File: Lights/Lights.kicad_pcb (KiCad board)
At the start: 2 copper layers, 102.5 x 200 mm, 100 parts, among them J101 chain_in, J102 chain_out, J103 Input1, J104 Input1, J105 Input1, J106 THRU, J107 THRU, J108 IN, J109 EuroPower, J110 ExternalPower, J401 Light, J701 Light, J801 Light, Q401 PN2222A, Q402 IRF540N, Q701 PN2222A, Q702 IRF540N, Q801 PN2222A, Q802 IRF540N, U101 L7805, U102 L7805, U201 TL074, U301 74LS04, U302 6N138, U401 6N138, U501 TL074, U601 TL074, U701 6N138, U801 6N138

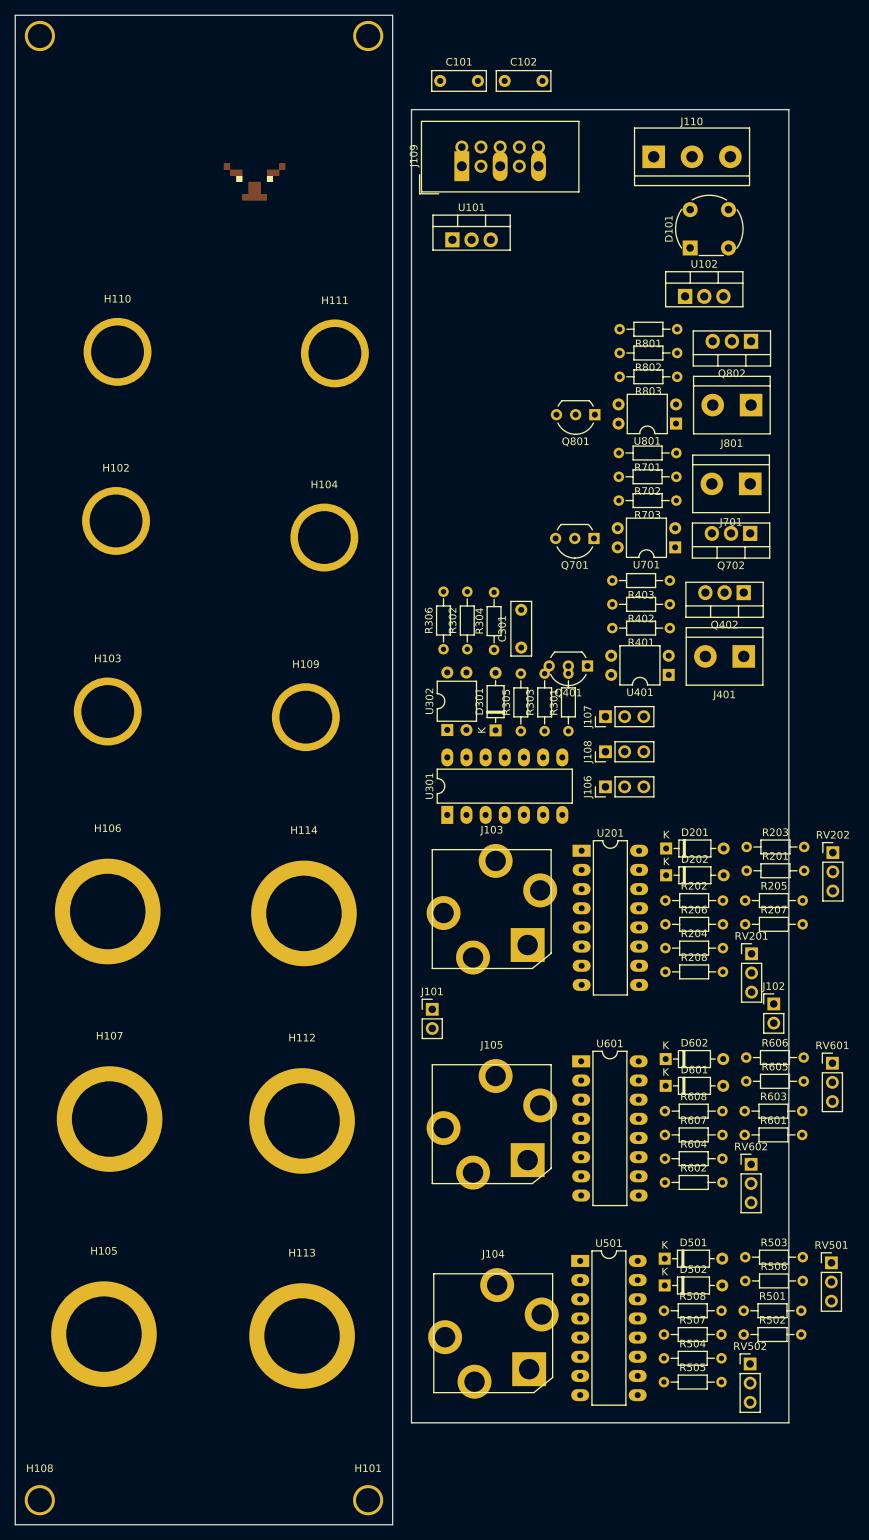
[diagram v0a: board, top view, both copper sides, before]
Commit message: Finished schematic and routing
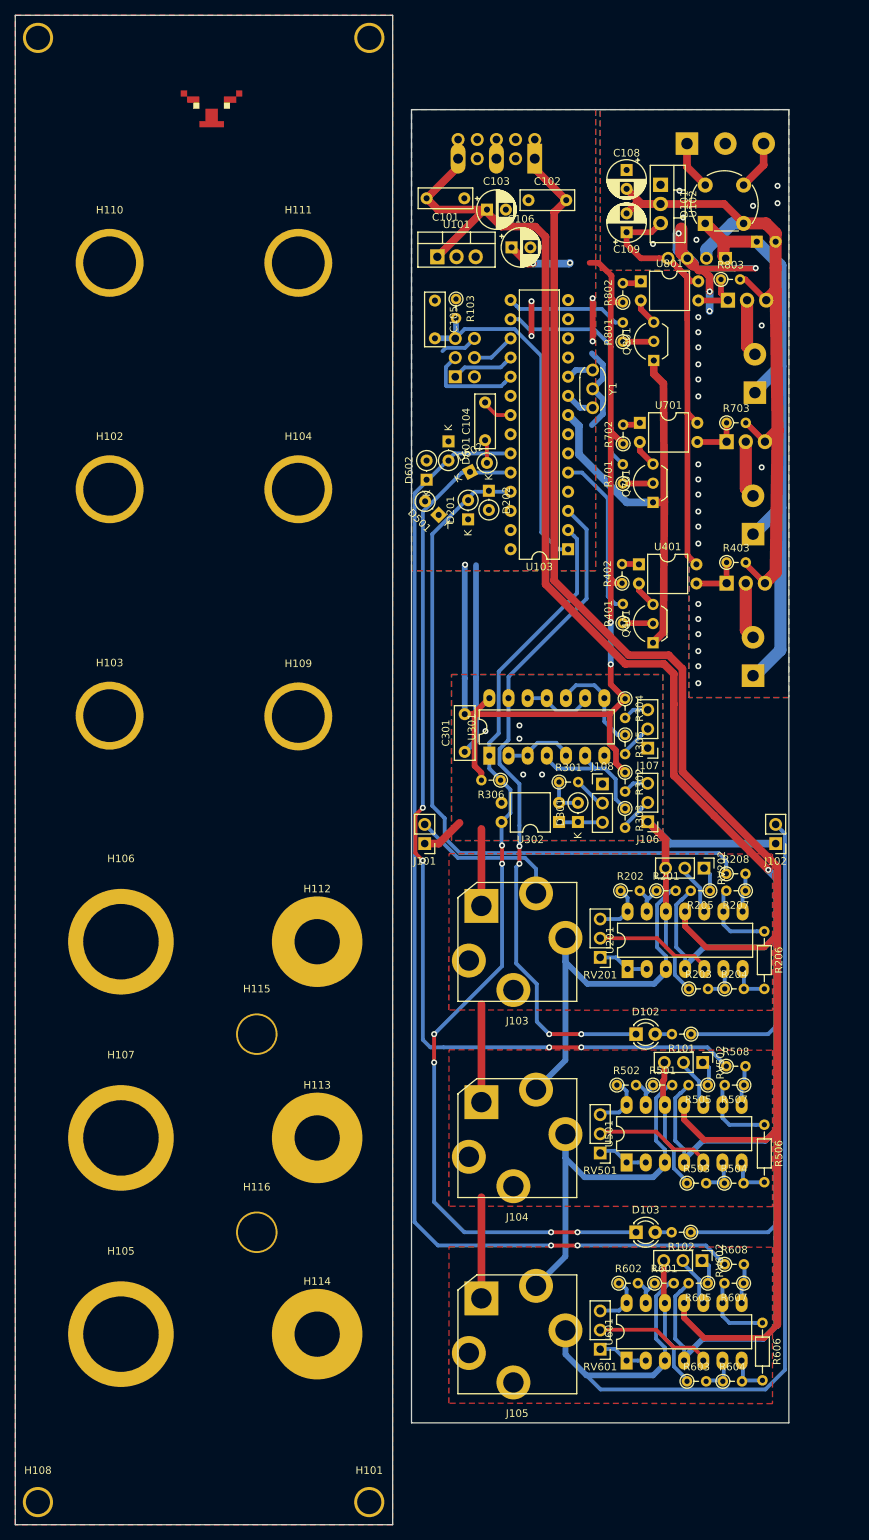
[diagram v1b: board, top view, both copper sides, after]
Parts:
- added C103: 1u, Capacitor_THT:CP_Radial_D5.0mm_P2.50mm, F.Cu at (74.5, 37.8)
- added C104: 100n, Capacitor_THT:C_Disc_D7.0mm_W2.5mm_P5.00mm, F.Cu at (74.2, 68.3)
- added C105: 100n, Capacitor_THT:C_Disc_D7.0mm_W2.5mm_P5.00mm, F.Cu at (67.6, 49.8)
- added C106: 1u, Capacitor_THT:CP_Radial_D5.0mm_P2.50mm, F.Cu at (77.8, 42.8)
- added C107: 10u, Capacitor_THT:CP_Radial_D5.0mm_P2.50mm, B.Cu at (110.2, 42.0)
- added C108: 1u, Capacitor_THT:CP_Radial_D5.0mm_P2.50mm, F.Cu at (93.0, 32.5)
- added C109: 1u, Capacitor_THT:CP_Radial_D5.0mm_P2.50mm, F.Cu at (93.0, 40.8)
- added D102: LED, LED_THT:LED_D3.0mm_FlatTop, F.Cu at (94.2, 147.0)
- added D103: LED, LED_THT:LED_D3.0mm_FlatTop, F.Cu at (94.2, 173.2)
- added H115: Led_Hole, Kosmo_panel:Kosmo_LED_Hole, F.Cu at (44.0, 147.0)
- added H116: Led_Hole, Kosmo_panel:Kosmo_LED_Hole, F.Cu at (44.0, 173.2)
- added J111: Programming, Connector_IDC:IDC-Header_2x03_P2.54mm_Vertical, B.Cu at (70.3, 59.9)
- added J112: chain_power, Connector_PinHeader_2.54mm:PinHeader_1x04_P2.54mm_Vertical, B.Cu at (106.1, 44.2)
- added R101: 1K, Resistor_THT:R_Axial_DIN0204_L3.6mm_D1.6mm_P2.54mm_Vertical, F.Cu at (101.5, 147.0)
- added R102: 1K, Resistor_THT:R_Axial_DIN0204_L3.6mm_D1.6mm_P2.54mm_Vertical, F.Cu at (101.5, 173.2)
- added R103: 22k, Resistor_THT:R_Axial_DIN0204_L3.6mm_D1.6mm_P2.54mm_Vertical, F.Cu at (70.4, 49.6)
- added U103: ATmega328P-PU, Package_DIP:DIP-28_W7.62mm, F.Cu at (85.2, 82.8)
- added Y1: 16MHz, Crystal:Resonator-3Pin_W6.0mm_H3.0mm, F.Cu at (88.5, 59.0)
- D201, D202, D301, D501, D502, D601, D602: footprint Diode_THT:D_DO-35_SOD27_P7.62mm_Horizontal -> Diode_THT:D_DO-35_SOD27_P2.54mm_Vertical_KathodeUp
- H112, H113, H114: footprint Kosmo_panel:Kosmo_Jack_Hole -> MountingHole:MountingHole_6mm_Pad
- J104: value Input1 -> Input2
- J105: value Input1 -> Input3
- J107: value THRU -> OUT
- J109, J110, J401, J701, J801, Q402, Q702, Q802: moved to B.Cu
- R201, R202, R203, R204, R205, R207, R208, R301, R302, R303, R304, R305, R306, R401, R402, R403, R501, R502, R503, R504, R505, R507, R508, R601, R602, R603, R604, R605, R607, R608, R701, R702, R703, R801, R802, R803: footprint Resistor_THT:R_Axial_DIN0204_L3.6mm_D1.6mm_P7.62mm_Horizontal -> Resistor_THT:R_Axial_DIN0204_L3.6mm_D1.6mm_P2.54mm_Vertical
- U201, U501, U601: footprint Package_DIP:DIP-16_W7.62mm_LongPads -> Package_DIP:DIP-14_W7.62mm_LongPads
- moved D502 110.8 mm to (72.2, 72.5), turned to 28 degrees
- moved D501 103.0 mm to (68.1, 78.2), turned to 135 degrees
- moved D601 90.1 mm to (69.4, 68.5), turned to 270 degrees
- moved D602 83.0 mm to (66.5, 73.5), turned to 90 degrees
- moved D202 56.1 mm to (74.8, 75.0), turned to 270 degrees
- moved H114 55.8 mm to (52.0, 186.8)
- moved D201 50.9 mm to (72.0, 78.8), turned to 90 degrees
- moved RV601 48.8 mm to (89.5, 188.8), turned to 180 degrees
- moved RV502 40.4 mm to (103.1, 150.8), turned to 270 degrees
- moved U601 40.1 mm to (93.0, 190.2), turned to 90 degrees
- moved R505 39.8 mm to (103.8, 153.8), turned to 180 degrees
- moved R502 37.1 mm to (91.7, 153.8)
- moved R603 36.6 mm to (101.0, 193.0)
- moved R606 35.2 mm to (111.0, 185.2), turned to 270 degrees
- moved R507 34.7 mm to (108.5, 153.8), turned to 180 degrees
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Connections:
- net /Normalize/Norm renamed /ADC1
- net /sheet606D2594/Norm renamed /ADC2
- net /sheet606D67AE/Norm renamed /ADC3
- J106 pad R: Net-(J106-PadR) -> /MIDI/MIDI_THRU-
- J106 pad S: Net-(J106-PadS) -> GND
- J106 pad T: Net-(J106-PadT) -> /MIDI/MIDI_THRU+
- J107 pad R: Net-(J107-PadR) -> /MIDI/MIDI_OUT-
- J107 pad S: Net-(J107-PadS) -> GND
- J107 pad T: Net-(J107-PadT) -> /MIDI/MIDI_OUT+
- J108 pad R: Net-(J108-PadR) -> /MIDI/MIDI_IN-
- J108 pad T: Net-(J108-PadT) -> /MIDI/MIDI_IN+
- Q402 pad 1: +5V -> Net-(Q402-Pad1)
- Q702 pad 1: +5V -> Net-(Q702-Pad1)
- Q802 pad 1: +5V -> Net-(Q802-Pad1)
- R401 pad 2: /Switching/PWM -> /PWM3
- R403 pad 1: Net-(R403-Pad1) -> Net-(Q402-Pad1)
- R701 pad 2: /sheet60725942/PWM -> /PWM2
- R703 pad 1: Net-(R703-Pad1) -> Net-(Q702-Pad1)
- R801 pad 2: /sheet607266DD/PWM -> /PWM1
- R803 pad 1: Net-(R803-Pad1) -> Net-(Q802-Pad1)
- U401 pad 3: Net-(R403-Pad1) -> Net-(Q402-Pad1)
- U401 pad 4: +5V -> +5VP
- U701 pad 3: Net-(R703-Pad1) -> Net-(Q702-Pad1)
- U701 pad 4: +5V -> +5VP
- U801 pad 3: Net-(R803-Pad1) -> Net-(Q802-Pad1)
- U801 pad 4: +5V -> +5VP
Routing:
- net +12V: track 0.00 -> 299.3 mm, vias 0 -> 1
- net GND: track 0.00 -> 233.3 mm, vias 0 -> 9
- net -12V: track 0.00 -> 223.3 mm
- net /ADC3: track 0.00 -> 154.9 mm, vias 0 -> 2
- net +5V: track 0.00 -> 140.3 mm, vias 0 -> 5
- net /sheet606D67AE/In: track 0.00 -> 135.7 mm
- net /MIDI_IN: track 0.00 -> 128.2 mm, vias 0 -> 6
- net /ADC2: track 0.00 -> 127.0 mm, vias 0 -> 4
- net -VDC: track 0.00 -> 97.7 mm
- net /ADC1: track 0.00 -> 93.9 mm
- net /MIDI_OUT: track 0.00 -> 89.7 mm, vias 0 -> 4
- net +VDC: track 0.00 -> 80.2 mm
- net +5VP: track 0.00 -> 62.0 mm
- net /Normalize/In: track 0.00 -> 52.7 mm
- net /sheet606D2594/In: track 0.00 -> 52.4 mm
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- added copper zone on F.Cu, net +5V
- added copper zone on B.Cu, net GND
- added copper zone on F.Cu, net GND
- added copper zone on B.Cu, net GNDPWR
- added copper zone on F.Cu, net GNDPWR
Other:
- net class Default: clearance 0.2 -> 0.127; trace_width 0.25 -> 0.127; via_dia 0.8 -> 0.6858; via_drill 0.4 -> 0.3302
- rule trace_clearance: 0.2 -> 0.127
- rule trace_min: 0.2 -> 0.127
- rule via_min_drill: 0.3 -> 0.2
- rule via_min_size: 0.4 -> 0.45
